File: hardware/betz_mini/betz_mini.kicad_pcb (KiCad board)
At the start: 4 copper layers, 40 x 40 mm, 60 parts, among them J1 upstream, J2 downstream, J3 ARM SWD, J4 BLDC, J5 BONUS, U1 stm32g474ceu6, U2 AS5047U, U3 IIS328DQ, U4 MP6540, U5 LMZM23601V3, U6 THVD2450, X1 8 MHz

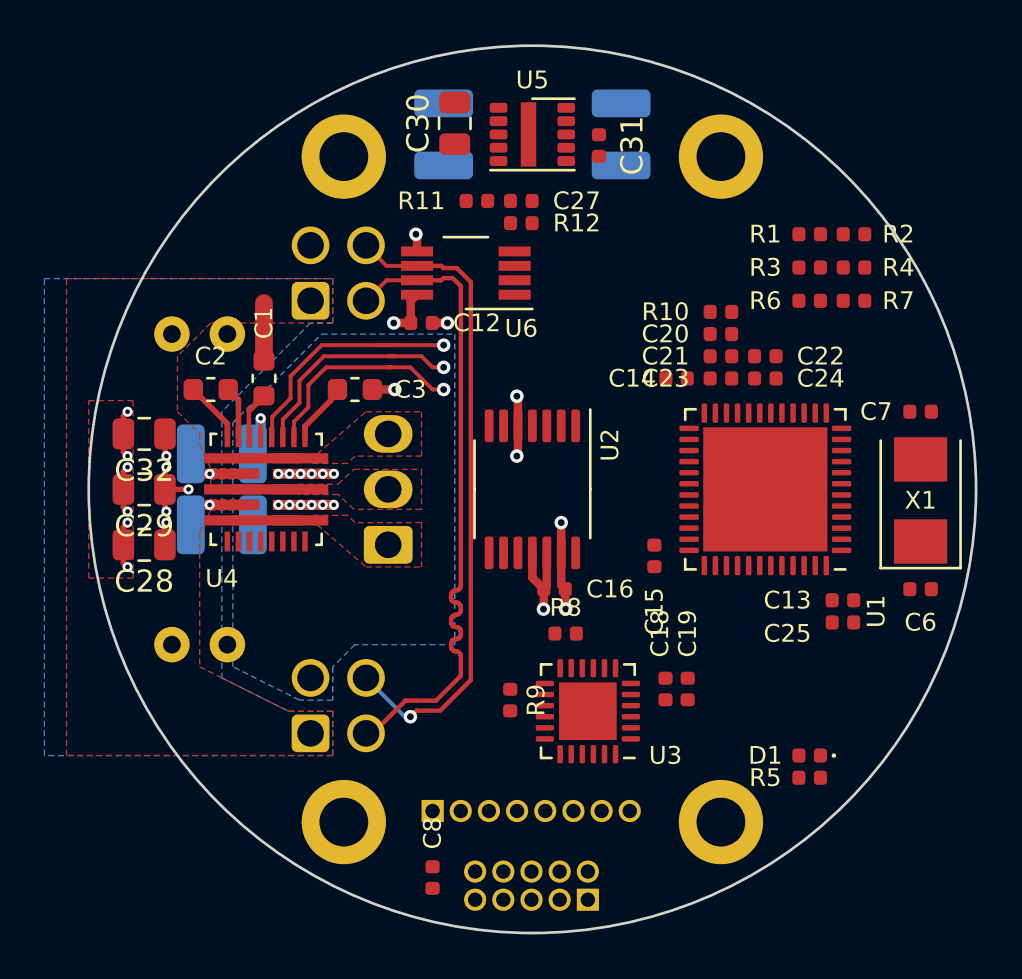
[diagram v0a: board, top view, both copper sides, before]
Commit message: rev.A first pass complete
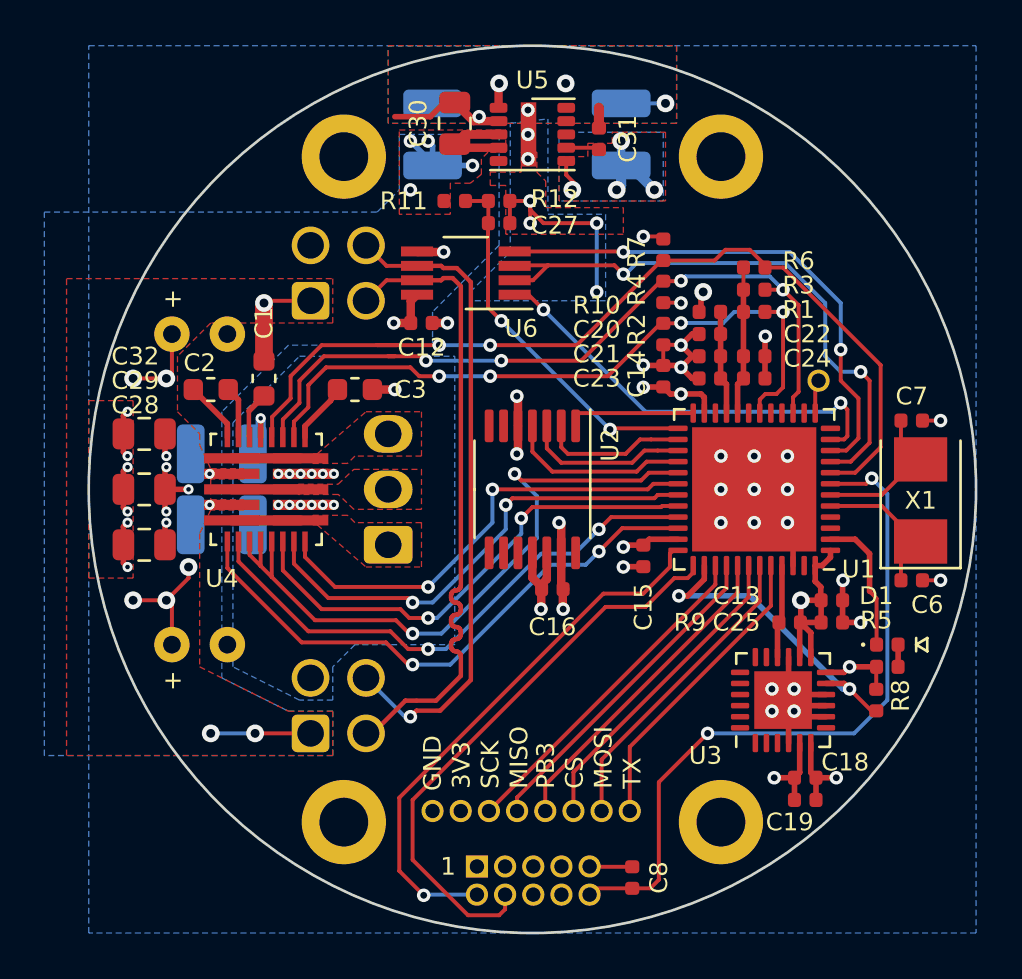
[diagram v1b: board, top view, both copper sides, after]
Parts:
- added J6: EXTRA_BONUS, Connector_PinHeader_1.27mm:PinHeader_1x01_P1.27mm_Vertical, B.Cu at (162.9, 95.1)
- added LOGO1: Logo_Open_Hardware_Small, Symbol:OSHW-Logo_7.5x8mm_SilkScreen, B.Cu at (160.2, 100.0)
- moved R8 14.3 mm to (165.5, 109.5), turned to -90 degrees
- moved R9 13.1 mm to (161.6, 106.0), turned to 180 degrees
- moved R2 9.71 mm to (155.9, 93.0), turned to -90 degrees
- moved C8 9.00 mm to (154.5, 117.5), turned to 90 degrees
- moved R7 8.90 mm to (155.9, 89.2), turned to 90 degrees
- moved U3 8.81 mm to (161.3, 109.5), turned to 90 degrees
- moved R4 8.67 mm to (155.9, 91.1), turned to -90 degrees
- moved C18 7.46 mm to (162.3, 113.0), turned to 0 degrees
- moved C19 7.29 mm to (162.3, 114.0), turned to 0 degrees
- moved D1 6.10 mm to (166.0, 107.0), turned to 0 degrees
- moved R5 6.10 mm to (166.0, 108.0), turned to 180 degrees
- moved J3 5.22 mm to (147.5, 117.0), turned to -90 degrees
- moved R1 4.30 mm to (160.0, 92.0)
- moved R6 2.92 mm to (160.0, 90.0)
- moved R3 2.69 mm to (160.0, 91.0)
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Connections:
- J5 pad 3: /DEBUG_TX -> /BONUS_SCK
- J5 pad 4: /BONUS_MOSI -> /BONUS_MISO
- J5 pad 5: /BONUS_MISO -> /BONUS_GPIO
- J5 pad 6: /BONUS_SCK -> /BONUS_CS
- J5 pad 7: /BONUS_GPIO -> /BONUS_MOSI
- J5 pad 8: /BONUS_CS -> /DEBUG_TX
- U1 pad 13: Net-(U1-Pad13) -> /PA5
- U1 pad 2: Net-(U1-Pad2) -> /STATUS_LED
- U1 pad 47: /STATUS_LED -> Net-(U1-Pad47)
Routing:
- net GND: track 21.3 -> 88.7 mm, vias 26 -> 62
- net /NRST: track 0.00 -> 31.9 mm, vias 0 -> 2
- net +3V3: track 6.61 -> 37.9 mm, vias 2 -> 13
- net /BLDC_EN: track 0.00 -> 30.4 mm, vias 0 -> 2
- net /IC: track 11.5 -> 41.6 mm, vias 1 -> 2
- net /RS485_DE: track 0.00 -> 26.7 mm, vias 0 -> 2
- net /SWCLK: track 0.00 -> 25.9 mm
- net /FAULT: track 0.00 -> 25.9 mm, vias 0 -> 2
- net VBUS: track 9.78 -> 35.0 mm, vias 7 -> 19
- net /SLEEP: track 0.00 -> 24.8 mm, vias 0 -> 2
- net /SWDIO: track 0.00 -> 24.8 mm, vias 0 -> 1
- net /IB: track 10.3 -> 34.1 mm, vias 1 -> 4
- net /RS485_DI: track 0.00 -> 23.6 mm, vias 0 -> 2
- net /PWMA: track 0.00 -> 22.5 mm, vias 0 -> 2
- net /IA: track 9.64 -> 31.7 mm, vias 1 -> 4
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- added copper zone on B.Cu, net +3V3
- added copper zone on F.Cu, net +3V3
- added copper zone on In2.Cu, net +3V3
- added copper zone on In2.Cu, net GND
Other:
- net class Default: clearance 0.2 -> 0.1524
- rule trace_clearance: 0.2 -> 0.1524
- board text added: "+24V-"
- board text added: "3V3"
- board text added: "A"
- board text added: "B"
- board text added: "BETZ MINI REV A MAY 2020"
- board text added: "CS"
- board text added: "GND"
- board text added: "MISO"
- board text added: "MOSI"
- board text added: "PB3"
- board text added: "SCK"
- board text added: "TX"
